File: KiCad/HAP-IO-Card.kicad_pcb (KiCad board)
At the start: 2 copper layers, 110 x 72 mm, 229 parts, among them CON601 AVR-JTAG-10, J201 TE_Connectivity_1-282834-0, J202 TE_Connectivity_282834-6, J203 GS3, J204 GS3, J205 GS3, J206 GS3, J207 GS3, J208 GS3, J209 GS3, J210 GS3, J211 TE_Connectivity_282834-6, J212 TE_Connectivity_1-282834-0, J401 TE_Connectivity_1-282834-0, J402 TE_Connectivity_282834-6, J501 TE_Connectivity_282834-3, J502 CONN_01X03_FEMALE, J601 ISP0, J602 ISP1, J603 CONN_01X02, J604 CONN_01X02, J605 CONN_01X02, J606 CONN_01X02, J607 CONN_01X03, J608 CONN_01X03, J701 5V_I/O_2, J702 5V_I/O_1, J703 NEO1, J704 NEO2, J705 NEO3, J706 NEO4, J707 CONN_01X03, Q201 ZXTN25050DFHTA, Q202 ZXTN25050DFHTA, Q203 ZXTN25050DFHTA, Q204 ZXTN25050DFHTA, Q205 ZXTN25050DFHTA, Q206 ZXTN25050DFHTA, Q207 ZXTN25050DFHTA, Q208 ZXTN25050DFHTA, U201 LTV-354T, U202 LTV-354T, U203 LTV-354T, U204 LTV-354T, U205 LTV-354T, U206 LTV-354T, U207 LTV-354T, U208 LTV-354T, U209 MCP23017, U401 ADS1115IDGST, U402 ADS1115IDGST, U501 LM1086-5V, U502 LM1086-3.3V, U701 TXB0102DCT

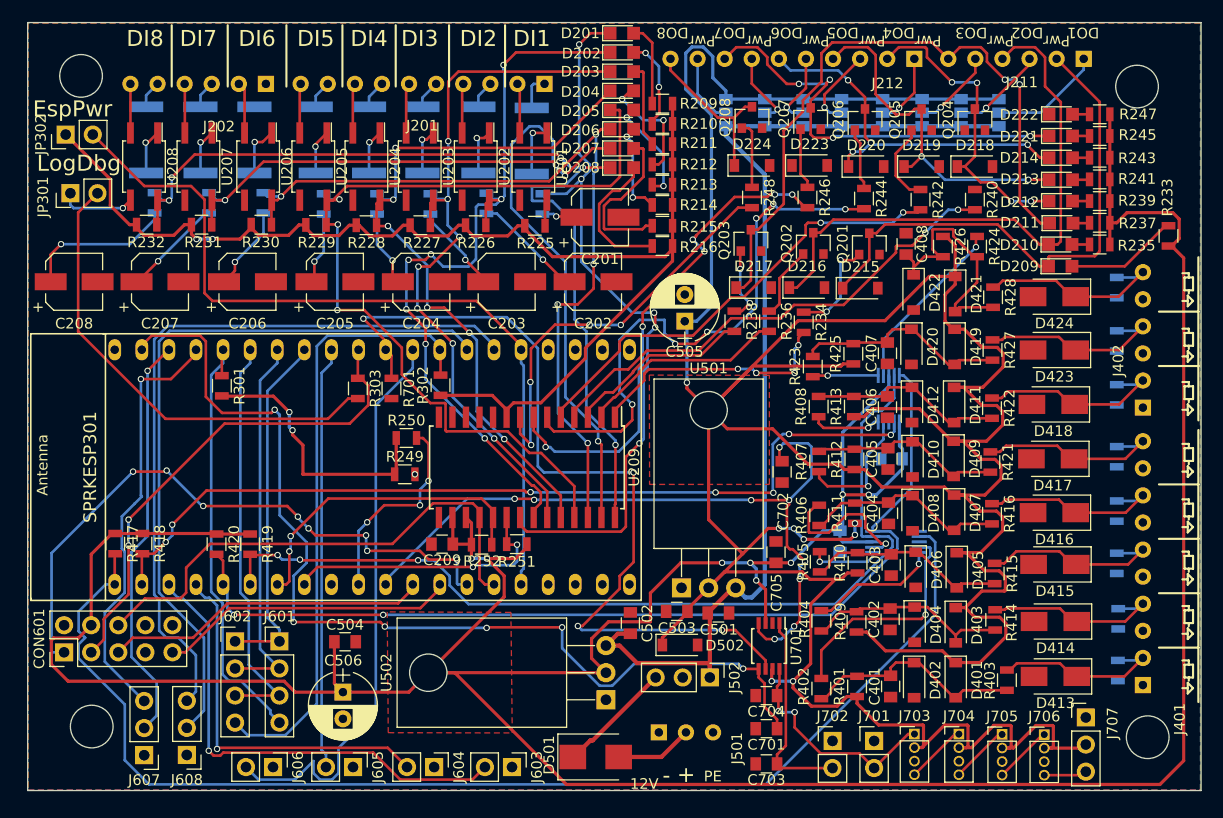
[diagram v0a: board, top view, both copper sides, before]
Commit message: Starting another routing pass
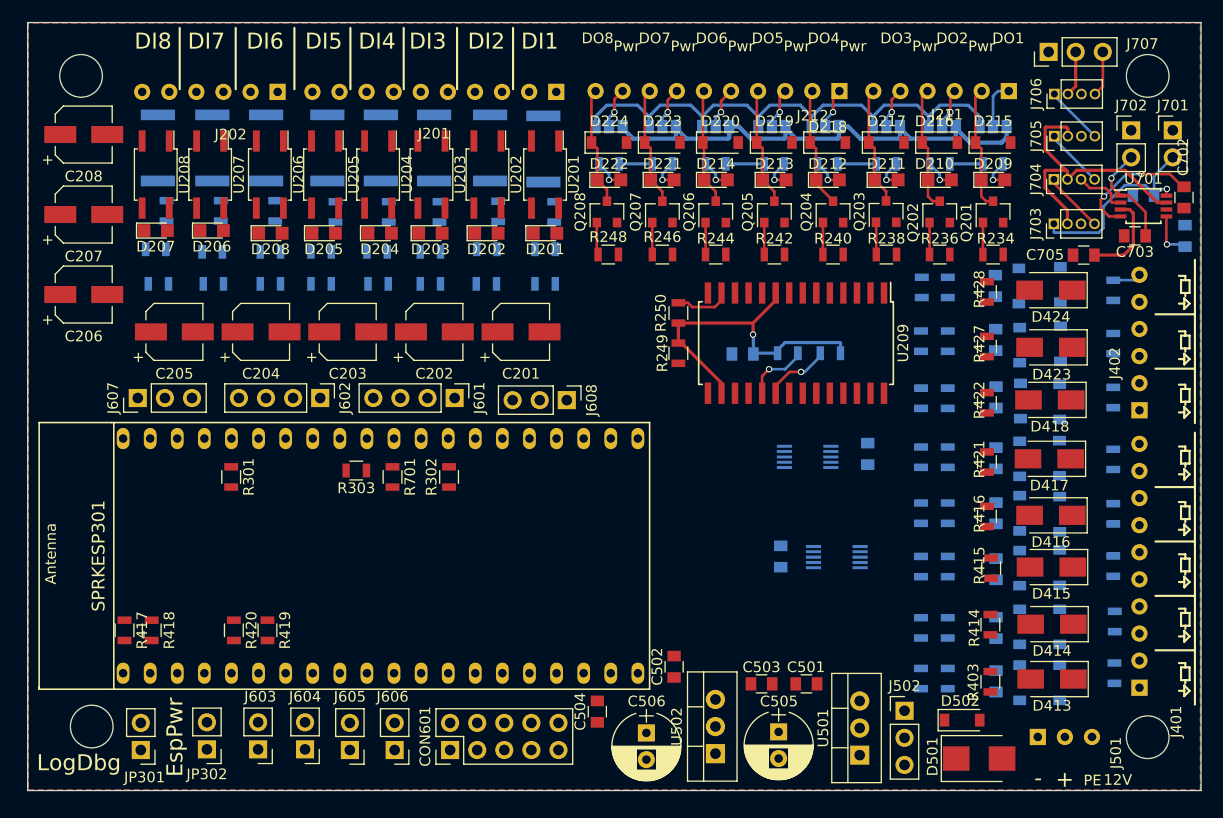
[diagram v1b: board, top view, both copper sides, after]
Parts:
- C209, C401, C402, C403, C404, C405, C406, C407, C408, C701, C704, D401, D402, D403, D404, D405, D406, D407, D408, D409, D410, D411, D412, D419, D420, D421, D422, R209, R210, R211, R212, R213, R214, R215, R216, R225, R226, R227, R228, R229, R230, R231, R232, R233, R235, R237, R239, R241, R243, R245, R247, R251, R252, R401, R402, R404, R405, R406, R407, R408, R409, R410, R411, R412, R413, R423, R424, R425, R426: moved to B.Cu
- U501, U502: footprint TO_SOT_Packages_THT:TO-220_Horizontal -> TO_SOT_Packages_THT:TO-220_Vertical
- moved J701 63.7 mm to (144.6, 27.6)
- moved J702 63.7 mm to (140.7, 27.6)
- moved J707 62.5 mm to (132.9, 20.2), turned to 90 degrees
- moved C701 60.6 mm to (145.7, 37.5), turned to 90 degrees
- moved C703 60.4 mm to (141.0, 37.5)
- moved J706 60.1 mm to (133.5, 24.2), turned to 90 degrees
- moved JP302 59.1 mm to (54.0, 85.6), turned to 180 degrees
- moved C704 58.7 mm to (141.8, 33.7)
- moved J705 56.3 mm to (133.5, 28.1), turned to 90 degrees
- moved U701 54.2 mm to (141.8, 34.7), turned to 0 degrees
- moved J704 52.8 mm to (133.4, 32.2), turned to 90 degrees
- moved JP301 52.6 mm to (47.8, 85.7), turned to 180 degrees
- moved J703 49.6 mm to (133.4, 36.3), turned to 90 degrees
- moved J608 48.7 mm to (87.8, 52.9), turned to 270 degrees
- moved R216 47.5 mm to (49.2, 38.7)
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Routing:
- net POWER3V3: track 474.9 -> 53.6 mm, vias 12 -> 1
- net POWER5V: track 360.5 -> 82.8 mm, vias 8 -> 0
- net SENSE_RDY_1: track 116.0 -> 0.00 mm
- net SENSE_SCL: track 91.9 -> 0.00 mm, vias 2 -> 0
- net 5V_I/O_1: track 95.7 -> 4.43 mm, vias 6 -> 1
- net DI7: track 90.7 -> 0.00 mm, vias 4 -> 0
- net DI8: track 90.6 -> 0.00 mm, vias 5 -> 0
- net SENSE_SDA: track 88.5 -> 0.00 mm, vias 3 -> 0
- net DI5: track 85.6 -> 0.00 mm, vias 3 -> 0
- net SENSE_RDY_2: track 83.0 -> 0.00 mm, vias 7 -> 0
- net 5V_I/O_Enable: track 81.1 -> 0.00 mm, vias 4 -> 0
- net DI6: track 78.3 -> 0.00 mm, vias 5 -> 0
- net Net-(JP302-Pad2): track 76.1 -> 0.00 mm
- net DI2: track 73.2 -> 0.00 mm, vias 7 -> 0
- net DI1: track 72.2 -> 0.00 mm, vias 5 -> 0
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- removed copper zone on F.Cu, net POWER3V3
- removed copper zone on F.Cu, net POWER5V
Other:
- outline, holes or cut-outs redrawn
- board text added: "Out"
- board text removed: "Common"
